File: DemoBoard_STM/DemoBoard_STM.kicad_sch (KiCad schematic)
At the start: 56 parts, among them J1 USB4110GFA, J6 M55-7101242R, J7 MSD-1-A, J8 Conn_01x17_Pin, SW1 SW_Push, SW2 SW_Push, U1 RP2040, U2 W25Q128JVSIM, U3 MCP2518FDT-E_QBB, U4 TCAN332DCNR, U5 TLV75533PDBVR, Y1 ABM8-272-T3, Y2 ABM8-20.000MHZ-10-B1U-T

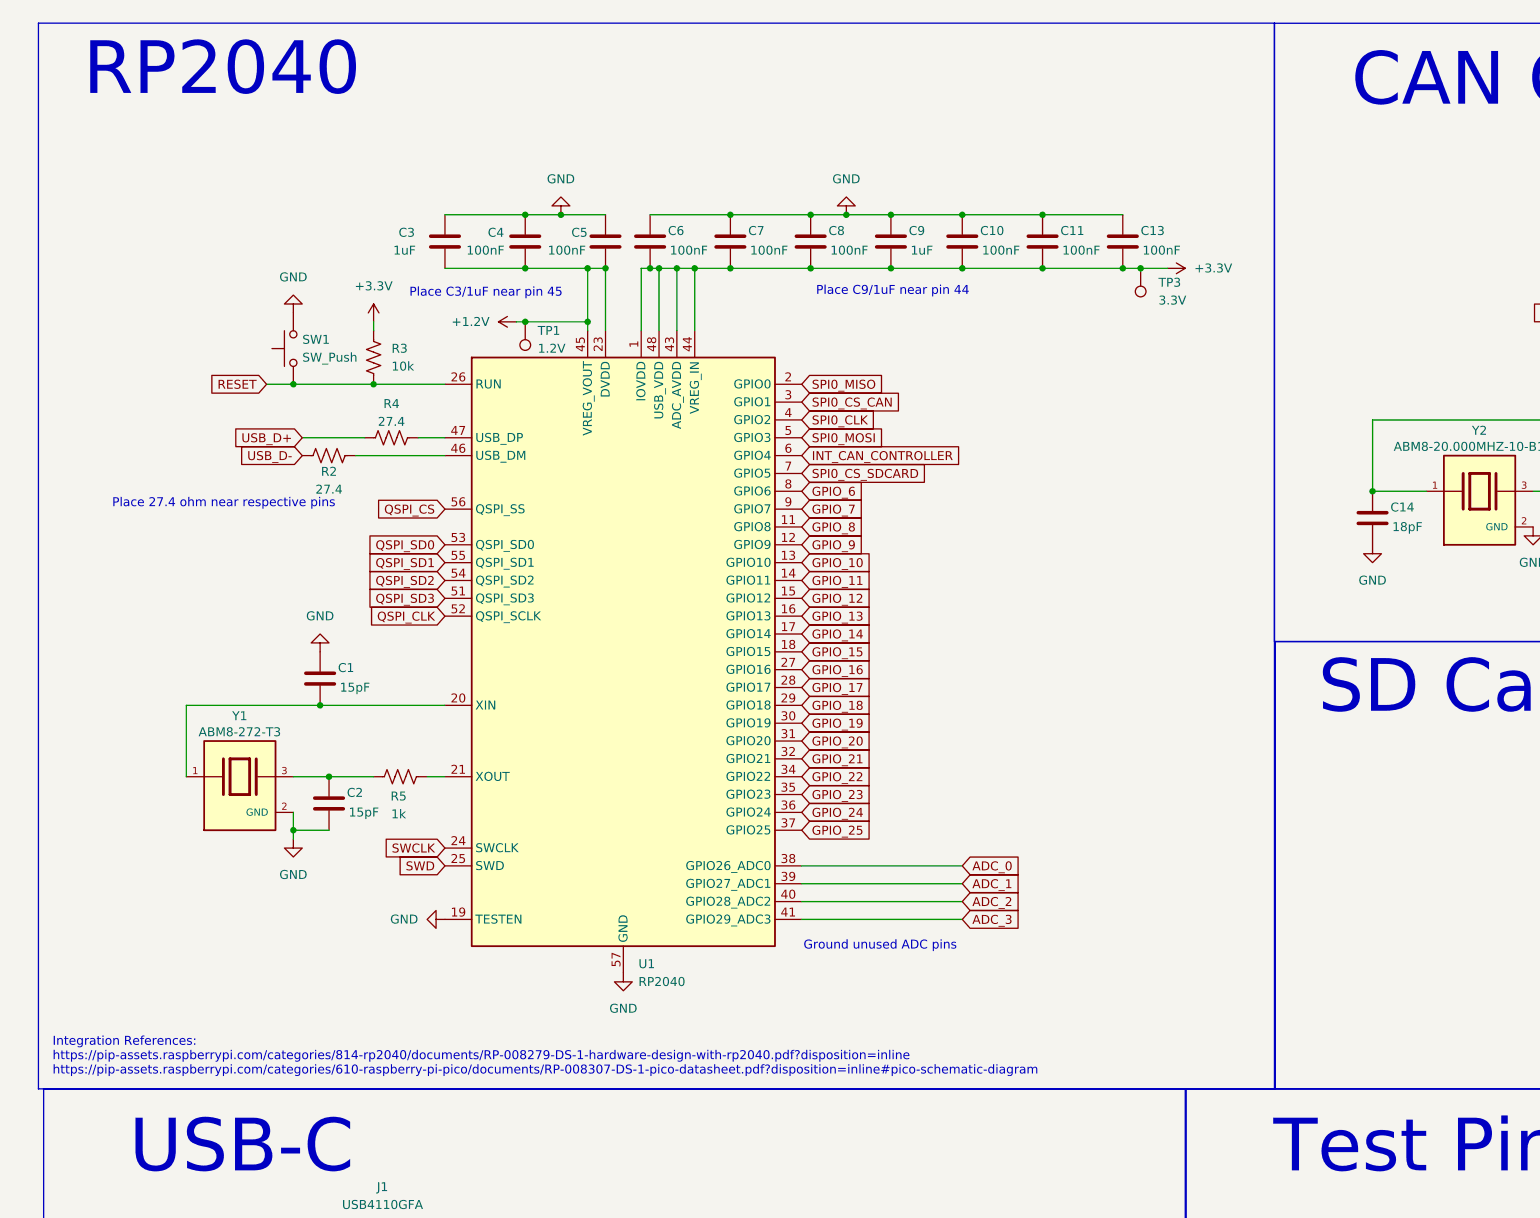
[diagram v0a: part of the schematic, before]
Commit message: Implement STM schematic
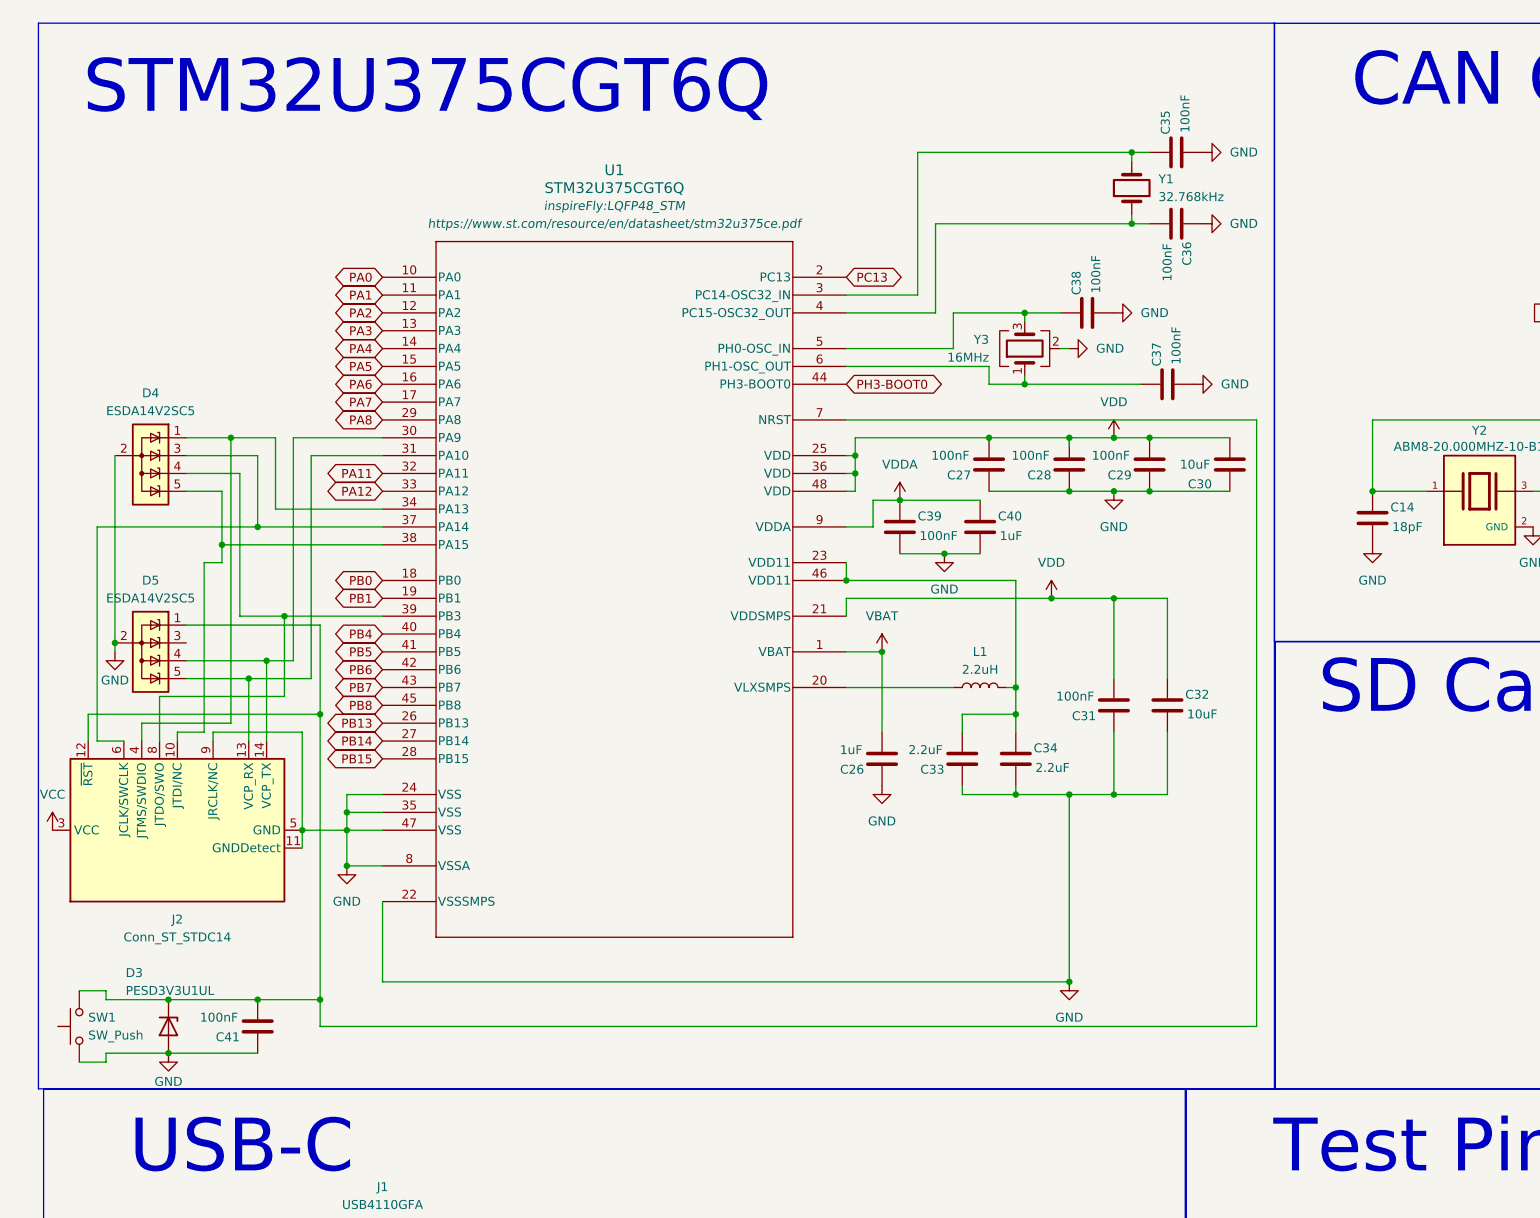
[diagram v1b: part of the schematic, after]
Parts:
- removed C1, C2: 15pF, Capacitor_SMD:C_0402_1005Metric_Pad0.74x0.62mm_HandSolder, symbol Device:C
- removed C10, C11, C13, C4, C5, C6, C7, C8: 100nF, Capacitor_SMD:C_0402_1005Metric_Pad0.74x0.62mm_HandSolder, symbol Device:C
- removed C3, C9: 1uF, Capacitor_SMD:C_0402_1005Metric_Pad0.74x0.62mm_HandSolder, symbol Device:C
- removed R2, R4: 27.4, Resistor_SMD:R_0402_1005Metric_Pad0.72x0.64mm_HandSolder, symbol Device:R_US
- removed R3: 10k, Resistor_SMD:R_0402_1005Metric_Pad0.72x0.64mm_HandSolder, symbol Device:R_US
- removed R5: 1k, Resistor_SMD:R_0402_1005Metric_Pad0.72x0.64mm_HandSolder, symbol Device:R_US
- removed TP1: 1.2V, TestPoint:TestPoint_Pad_D1.0mm, symbol Connector:TestPoint
- removed TP3: 3.3V, TestPoint:TestPoint_Pad_D1.0mm, symbol Connector:TestPoint
- removed U1: RP2040, Package_DFN_QFN:QFN-56-1EP_7x7mm_P0.4mm_EP3.2x3.2mm, symbol MCU_RaspberryPi:RP2040
- removed Y1: ABM8-272-T3, inspireFly:XTAL_ABM8-272-T3, symbol inspireFly:ABM8-272-T3
- added C26, C40: 1uF, Capacitor_SMD:C_0402_1005Metric_Pad0.74x0.62mm_HandSolder, symbol Device:C
- added C27, C28, C29, C31, C35, C36, C37, C38, C39, C41: 100nF, Capacitor_SMD:C_0402_1005Metric_Pad0.74x0.62mm_HandSolder, symbol Device:C
- added C30, C32: 10uF, Capacitor_SMD:C_0402_1005Metric_Pad0.74x0.62mm_HandSolder, symbol Device:C
- added C33, C34: 2.2uF, Capacitor_SMD:C_0402_1005Metric_Pad0.74x0.62mm_HandSolder, symbol Device:C
- added D3: PESD3V3U1UL, Diode_SMD:D_SOD-882, symbol Diode:PESD3V3U1UL
- added D4, D5: ESDA14V2SC5, Package_TO_SOT_SMD:SOT-23-5, symbol Power_Protection:ESDA14V2SC5
- added J2: Conn_ST_STDC14, symbol Connector:Conn_ST_STDC14
- added L1: 2.2uH, Inductor_SMD:L_0402_1005Metric_Pad0.77x0.64mm_HandSolder, symbol Device:L
- added U1: STM32U375CGT6Q, inspireFly:LQFP48_STM, symbol STM32U375:STM32U375CGT6Q
- added Y1: 32.768kHz, Crystal:Crystal_SMD_2012-2Pin_2.0x1.2mm_HandSoldering, symbol Device:Crystal
- added Y3: 16MHz, Crystal:Crystal_SMD_3225-4Pin_3.2x2.5mm_HandSoldering, symbol Device:Crystal_GND24
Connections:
- net RESET is gone; now on net COVER_GND: SW1.1
- net COVER_GND: now also C26.1, C27.1, C28.1, C29.1, C30.1, C31.1, C32.2, C33.1, C34.2, C35.2, C36.1, C37.2, C38.2, C39.2, C40.2, C41.1, D3.2 (A), D4.2 (A), D5.2 (A), J2.11 (GNDDetect), J2.5 (GND), J2.7 (GND), J2.9 (JRCLK/NC), U1.22 (VSSSMPS), U1.24 (VSS), U1.35 (VSS), U1.47 (VSS), U1.8 (VSSA), Y3.2 (G), Y3.4 (G); no longer SW1.2
- new net: C37.1, U1.6 (PH1-OSC_OUT), Y3.1
- new net: D4.5 (K), J2.10 (JTDI/NC), U1.38 (PA15)
- new net: C41.2, D3.1 (K), D5.1 (K), J2.12 (~{RST}), SW1.2, U1.7 (NRST)
- new net: D5.5 (K), J2.13 (VCP_RX), U1.31 (PA10)
- new net: D5.4 (K), J2.14 (VCP_TX), U1.30 (PA9)
- new net: D4.1 (K), J2.4 (JTMS/SWDIO), U1.34 (PA13)
- new net: D4.3 (K), J2.6 (JCLK/SWCLK), U1.37 (PA14)
- new net: D4.4 (K), J2.8 (JTDO/SWO), U1.39 (PB3)
- new net: L1.1, U1.20 (VLXSMPS)
- new net: C33.2, C34.1, L1.2, U1.23 (VDD11), U1.46 (VDD11)
- new net: C38.1, U1.5 (PH0-OSC_IN), Y3.3
- new net: C35.1, U1.3 (PC14-OSC32_IN), Y1.2
- new net: C36.2, U1.4 (PC15-OSC32_OUT), Y1.1
- new net PA0: U1.10 (PA0)
- new net PA1: U1.11 (PA1)
- new net PA11: U1.32 (PA11)
- new net PA12: U1.33 (PA12)
- new net PA2: U1.12 (PA2)
- new net PA3: U1.13 (PA3)
- new net PA4: U1.14 (PA4)
- new net PA5: U1.15 (PA5)
- new net PA6: U1.16 (PA6)
- new net PA7: U1.17 (PA7)
- new net PA8: U1.29 (PA8)
- new net PB0: U1.18 (PB0)
- new net PB1: U1.19 (PB1)
- new net PB13: U1.26 (PB13)
- new net PB14: U1.27 (PB14)
- new net PB15: U1.28 (PB15)
- new net PB4: U1.40 (PB4)
- new net PB5: U1.41 (PB5)
- new net PB6: U1.42 (PB6)
- new net PB7: U1.43 (PB7)
- new net PB8: U1.45 (PB8)
- new net PC13: U1.2 (PC13)
- new net PH3-BOOT0: U1.44 (PH3-BOOT0)
- new net VBAT: C26.2, U1.1 (VBAT)
- new net VCC: J2.3 (VCC)
- new net VDD: C27.2, C28.2, C29.2, C30.2, C31.2, C32.1, U1.21 (VDDSMPS), U1.25 (VDD), U1.36 (VDD), U1.48 (VDD)
- new net VDDA: C39.1, C40.1, U1.9 (VDDA)
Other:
- note added: "STM32U375CGT6Q"
- note removed: "Ground unused ADC pins"
- note removed: "Integration References: https://pip-assets.raspberrypi.com/categories/814-rp2040/documents/RP-008279-DS-1-hardware-design-with-rp2040.pdf?disposition=inline https://pip-assets.raspberrypi.com/categories/610-raspberry-pi-pico/documents/RP-008307-DS-1-pico-datasheet.pdf?disposition=inline#pico-schematic-diagram"
- note removed: "Place 27.4 ohm near respective pins"
- note removed: "Place C3/1uF near pin 45"
- note removed: "Place C9/1uF near pin 44"
- note removed: "RP2040"
